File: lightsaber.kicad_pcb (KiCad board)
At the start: 2 copper layers, 31 x 112.5 mm, 8 parts, among them SW1 Button, SW3 POWER, U1 C3 Pico

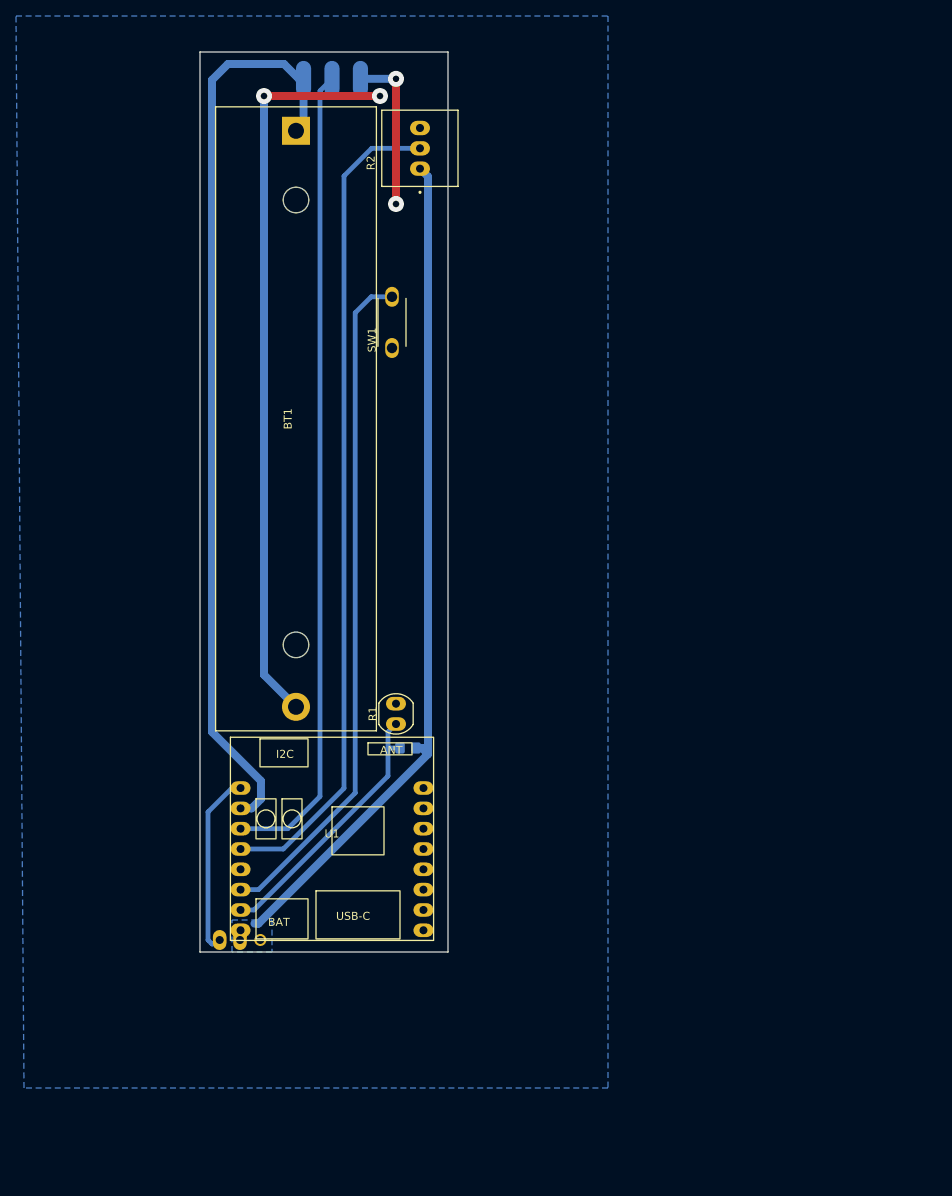
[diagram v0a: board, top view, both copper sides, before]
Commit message: Update PCB for Lightsaber
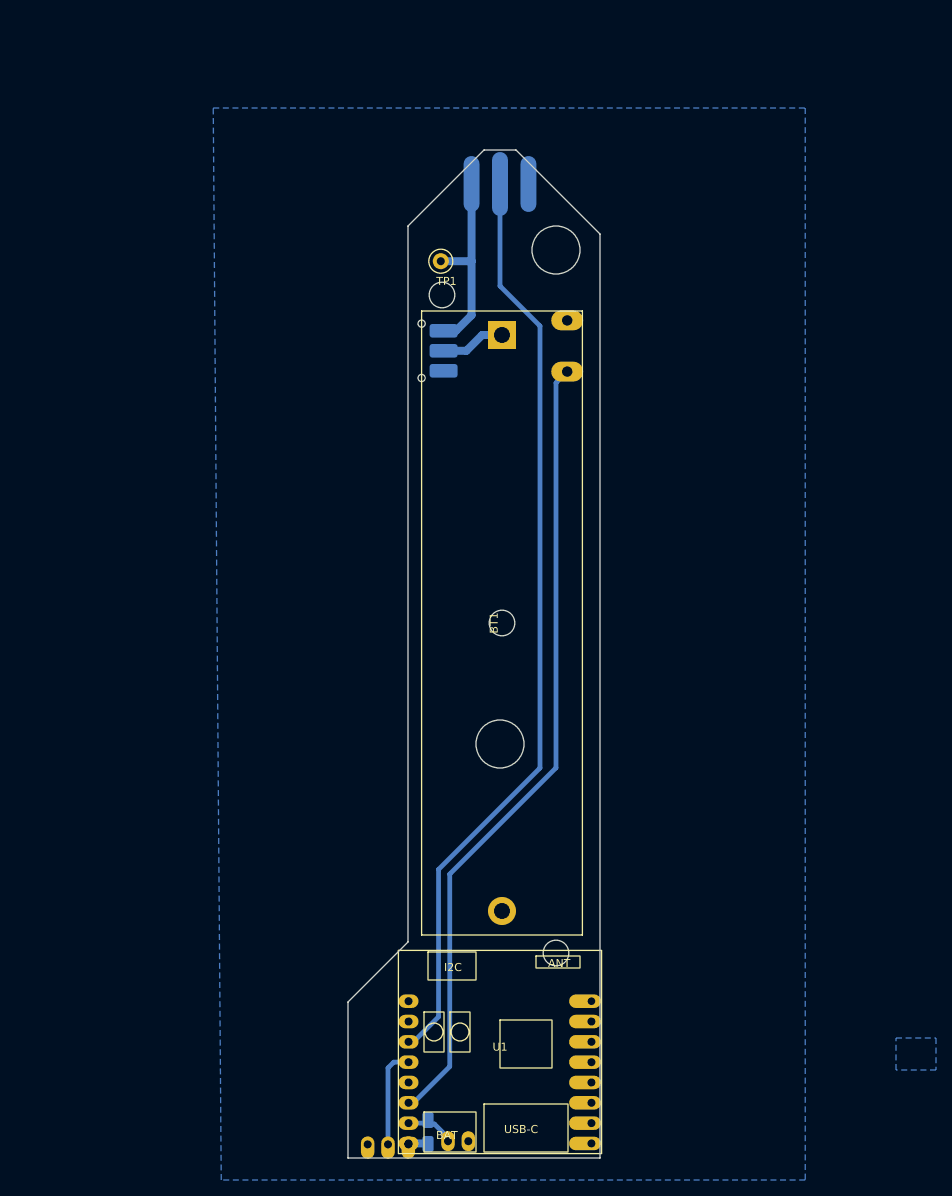
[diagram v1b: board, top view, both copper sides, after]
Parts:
- removed SW3: POWER, as12ap:as12ap
- added SW2: POWER, Button_Switch_SMD:SW_SPDT_CK_JS102011SAQN, B.Cu at (110.7, 59.9)
- added TP1: TO-BAT, TestPoint:TestPoint_Loop_D2.50mm_Drill1.0mm, F.Cu at (113.1, 48.6)
- R1, R2, SW1: moved to B.Cu
- moved R2 124.6 mm to (106.5, 159.1), turned to 180 degrees
- moved R1 52.6 mm to (114.0, 158.7), turned to 0 degrees
- moved R3 48.1 mm to (111.5, 157.5), turned to 90 degrees
- moved BT1 36.3 mm to (120.8, 57.9)
- moved U1 33.9 mm to (120.5, 147.5)
- moved NP1 24.8 mm to (120.5, 39.0)
- moved SW1 22.2 mm to (128.9, 56.0), turned to -90 degrees
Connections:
- BT1 pad 1: +4V -> VBAT
- U1 pad 15: +4V -> unconnected-(U1-IO3/VBAT-Pad15)
- U1 pad 16: Power -> unconnected-(U1-RST/EN-Pad16)
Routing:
- net GND: track 112.6 -> 0.00 mm, vias 4 -> 0
- net +3V3: track 110.2 -> 2.65 mm
- net +4V: track 115.4 -> 24.5 mm
- net Poti: track 103.5 -> 12.8 mm
- net Light: track 33.8 -> 6.13 mm
- net Power: track 23.0 -> 0.00 mm
- net Button: track 84.8 -> 100.0 mm
- net Neopixel: track 101.9 -> 116.5 mm
- net VBAT: track 0.00 -> 8.12 mm
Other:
- board size 31 x 112.5 mm -> 31.5 x 126 mm
